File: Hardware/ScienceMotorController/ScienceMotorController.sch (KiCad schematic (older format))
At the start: 0 parts

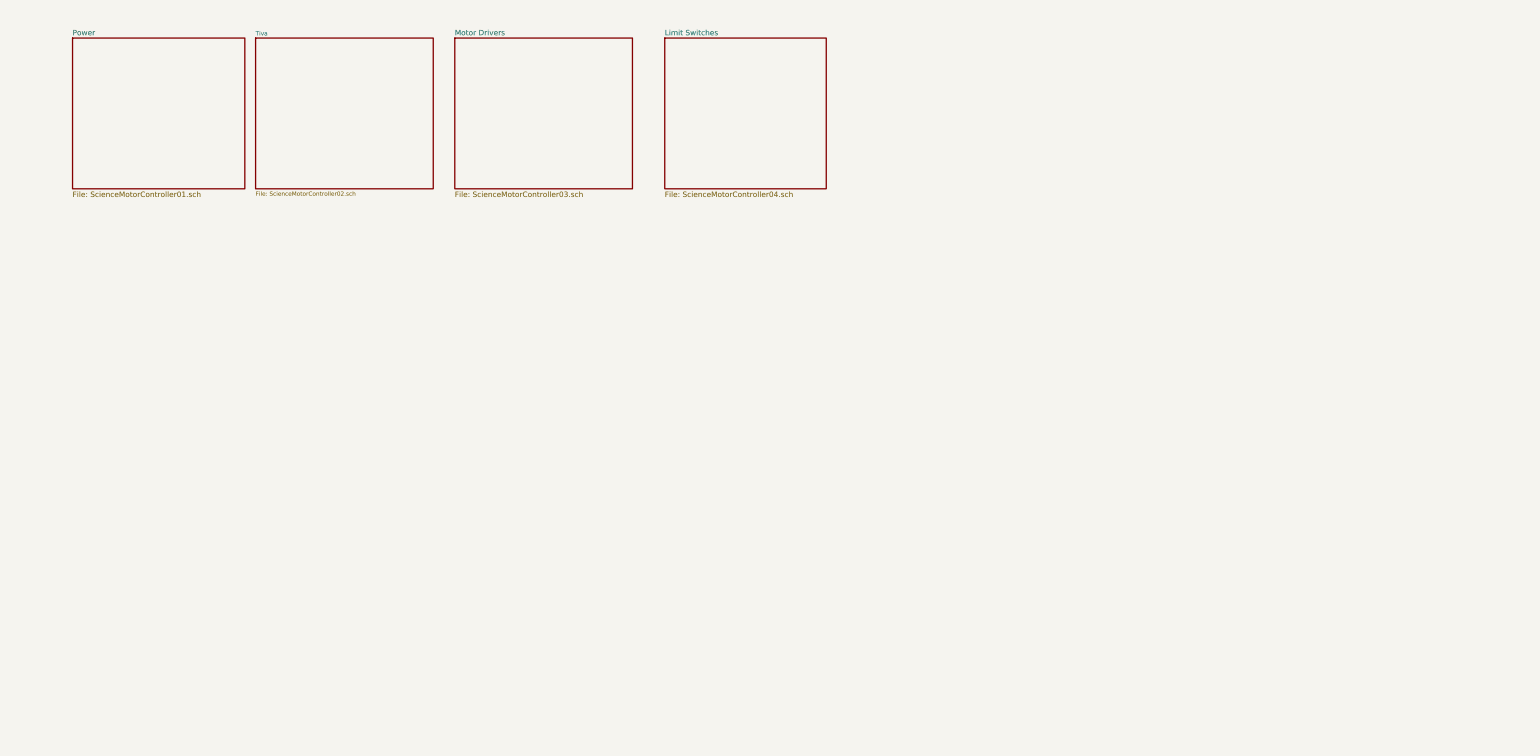
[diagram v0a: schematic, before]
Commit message: schematic review
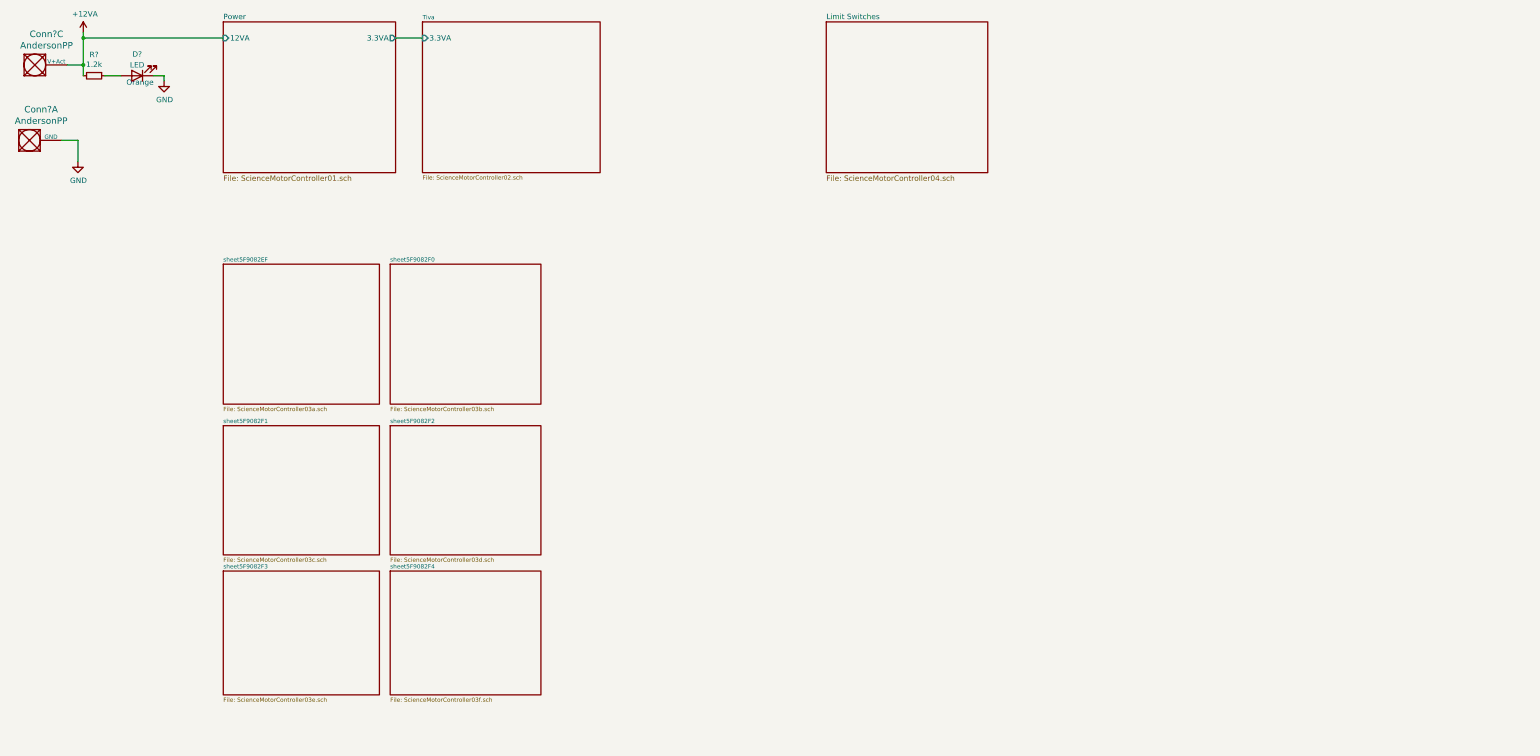
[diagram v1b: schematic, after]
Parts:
- added Conn? (x2): AndersonPP, symbol MRDT_Connectors:AndersonPP
- added D?: LED, symbol Device:LED
- added R?: 1.2k, symbol Device:R_Small
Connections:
- new net: D?.2 (A), R?.1
- new net +12VA: Conn?.3 (V+Act), R?.2
- new net GND: Conn?.1 (GND), D?.1 (K)
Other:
- note added: "Orange"
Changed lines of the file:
@@
 $Descr A 11000 8500
 encoding utf-8
-Sheet 1 11
+Sheet 1 10
 Title ""
 Date ""
@@
 $EndDescr
 $Sheet
-S 1100 1050 1600 1400
+S 2500 900  1600 1400
 U 5F6E1E86
 F0 "Power" 50
 F1 "ScienceMotorController01.sch" 50
+F2 "12VA" I L 2500 1050 50
+F3 "3.3VA" O R 4100 1050 50
 $EndSheet
 $Sheet
-S 2800 1050 1650 1400
+S 4350 900  1650 1400
 U 5F7148FA
 F0 "Tiva" 39
 F1 "ScienceMotorController02.sch" 39
+F2 "3.3VA" I L 4350 1050 50
 $EndSheet
 $Sheet
-S 4650 1050 1650 1400
-U 5F7D111E
-F0 "Motor Drivers" 50
-F1 "ScienceMotorController03.sch" 50
-$EndSheet
-$Sheet
-S 6600 1050 1500 1400
+S 8100 900  1500 1400
 U 5F81B171
 F0 "Limit Switches" 50
 F1 "ScienceMotorController04.sch" 50
 $EndSheet
+$Comp
+L MRDT_Connectors:AndersonPP Conn?
+U 3 1 5F8E3C0A
+P 650 1400
+AR Path="/5F6E1E86/5F8E3C0A" Ref="Conn?"  Part="3"
+AR Path="/5F8E3C0A" Ref="Conn?"  Part="3"
+F 0 "Conn?" H 858 1787 60  0000 C CNN
+F 1 "AndersonPP" H 858 1681 60  0000 C CNN
+F 2 "" H 500 850 60  0001 C CNN
+F 3 "" H 500 850 60  0001 C CNN
+	3    650  1400
+	1    0    0    -1
+$EndComp
+Wire Wire Line
+	1050 1300 1200 1300
+$Comp
+L power:+12VA #PWR?
+U 1 1 5F8E3C12
+P 1200 1000
+AR Path="/5F6E1E86/5F8E3C12" Ref="#PWR?"  Part="1"
+AR Path="/5F8E3C12" Ref="#PWR?"  Part="1"
+F 0 "#PWR?" H 1200 850 50  0001 C CNN
+F 1 "+12VA" H 1215 1173 50  0000 C CNN
+F 2 "" H 1200 1000 50  0001 C CNN
+F 3 "" H 1200 1000 50  0001 C CNN
+	1    1200 1000
+	1    0    0    -1
+$EndComp
+$Comp
+L Device:LED D?
+U 1 1 5F8E3C18
+P 1700 1400
+AR Path="/5F6E1E86/5F8E3C18" Ref="D?"  Part="1"
+AR Path="/5F8E3C18" Ref="D?"  Part="1"
+F 0 "D?" H 1700 1200 50  0000 C CNN
+F 1 "LED" H 1700 1300 50  0000 C CNN
+F 2 "" H 1700 1400 50  0001 C CNN
+F 3 "~" H 1700 1400 50  0001 C CNN
+	1    1700 1400
+	-1   0    0    1
+$EndComp
+Wire Wire Line
+	1200 1400 1200 1300
+Connection ~ 1200 1300
+$Comp
+L Device:R_Small R?
+U 1 1 5F8E3C20
+P 1300 1400
+AR Path="/5F6E1E86/5F8E3C20" Ref="R?"  Part="1"
+AR Path="/5F8E3C20" Ref="R?"  Part="1"
+F 0 "R?" V 1104 1400 50  0000 C CNN
+F 1 "1.2k" V 1195 1400 50  0000 C CNN
+F 2 "" H 1300 1400 50  0001 C CNN
+F 3 "~" H 1300 1400 50  0001 C CNN
+	1    1300 1400
+	0    1    1    0
+$EndComp
+Wire Wire Line
+	1400 1400 1550 1400
+$Comp
+L power:GND #PWR?
+U 1 1 5F8E3C27
+P 1950 1450
+AR Path="/5F6E1E86/5F8E3C27" Ref="#PWR?"  Part="1"
+AR Path="/5F8E3C27" Ref="#PWR?"  Part="1"
+F 0 "#PWR?" H 1950 1200 50  0001 C CNN
+F 1 "GND" H 1955 1277 50  0000 C CNN
+F 2 "" H 1950 1450 50  0001 C CNN
+F 3 "" H 1950 1450 50  0001 C CNN
+	1    1950 1450
+	1    0    0    -1
+$EndComp
+Wire Wire Line
+	1850 1400 1950 1400
+Wire Wire Line
+	1950 1400 1950 1450
+Text Notes 1600 1500 0    50   ~ 0
+Orange
+Wire Wire Line
+	1200 1050 1200 1300
+Wire Wire Line
+	2500 1050 1200 1050
+Connection ~ 1200 1050
+Wire Wire Line
+	1200 1000 1200 1050
+$Comp
+L MRDT_Connectors:AndersonPP Conn?
+U 1 1 5F8FDE30
+P 600 2100
+AR Path="/5F6E1E86/5F8FDE30" Ref="Conn?"  Part="1"
+AR Path="/5F8FDE30" Ref="Conn?"  Part="1"
+F 0 "Conn?" H 808 2487 60  0000 C CNN
+F 1 "AndersonPP" H 808 2381 60  0000 C CNN
+F 2 "" H 450 1550 60  0001 C CNN
+F 3 "" H 450 1550 60  0001 C CNN
+	1    600  2100
+	1    0    0    -1
+$EndComp
+$Comp
+L power:GND #PWR?
+U 1 1 5F8FDE36
+P 1150 2200
+AR Path="/5F6E1E86/5F8FDE36" Ref="#PWR?"  Part="1"
+AR Path="/5F8FDE36" Ref="#PWR?"  Part="1"
+F 0 "#PWR?" H 1150 1950 50  0001 C CNN
+F 1 "GND" H 1155 2027 50  0000 C CNN
+F 2 "" H 1150 2200 50  0001 C CNN
+F 3 "" H 1150 2200 50  0001 C CNN
+	1    1150 2200
+	1    0    0    -1
+$EndComp
+Wire Wire Line
+	1150 2200 1150 2000
+Wire Wire Line
+	1150 2000 1000 2000
+Wire Wire Line
+	4100 1050 4350 1050
+$Sheet
+S 2500 3150 1450 1300
+U 5F9082F6
+F0 "sheet5F9082EF" 39
+F1 "ScienceMotorController03a.sch" 39
+$EndSheet
+$Sheet
+S 4050 3150 1400 1300
+U 5F9082F8
+F0 "sheet5F9082F0" 39
+F1 "ScienceMotorController03b.sch" 39
+$EndSheet
+$Sheet
+S 2500 4650 1450 1200
+U 5F9082FA
+F0 "sheet5F9082F1" 39
+F1 "ScienceMotorController03c.sch" 39
+$EndSheet
+$Sheet
+S 4050 4650 1400 1200
+U 5F9082FC
+F0 "sheet5F9082F2" 39
+F1 "ScienceMotorController03d.sch" 39
+$EndSheet
+$Sheet
+S 2500 6000 1450 1150
+U 5F9082FE
+F0 "sheet5F9082F3" 39
+F1 "ScienceMotorController03e.sch" 39
+$EndSheet
+$Sheet
+S 4050 6000 1400 1150
+U 5F908300
+F0 "sheet5F9082F4" 39
+F1 "ScienceMotorController03f.sch" 39
+$EndSheet
 $EndSCHEMATC

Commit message: made some more hierarchal changes
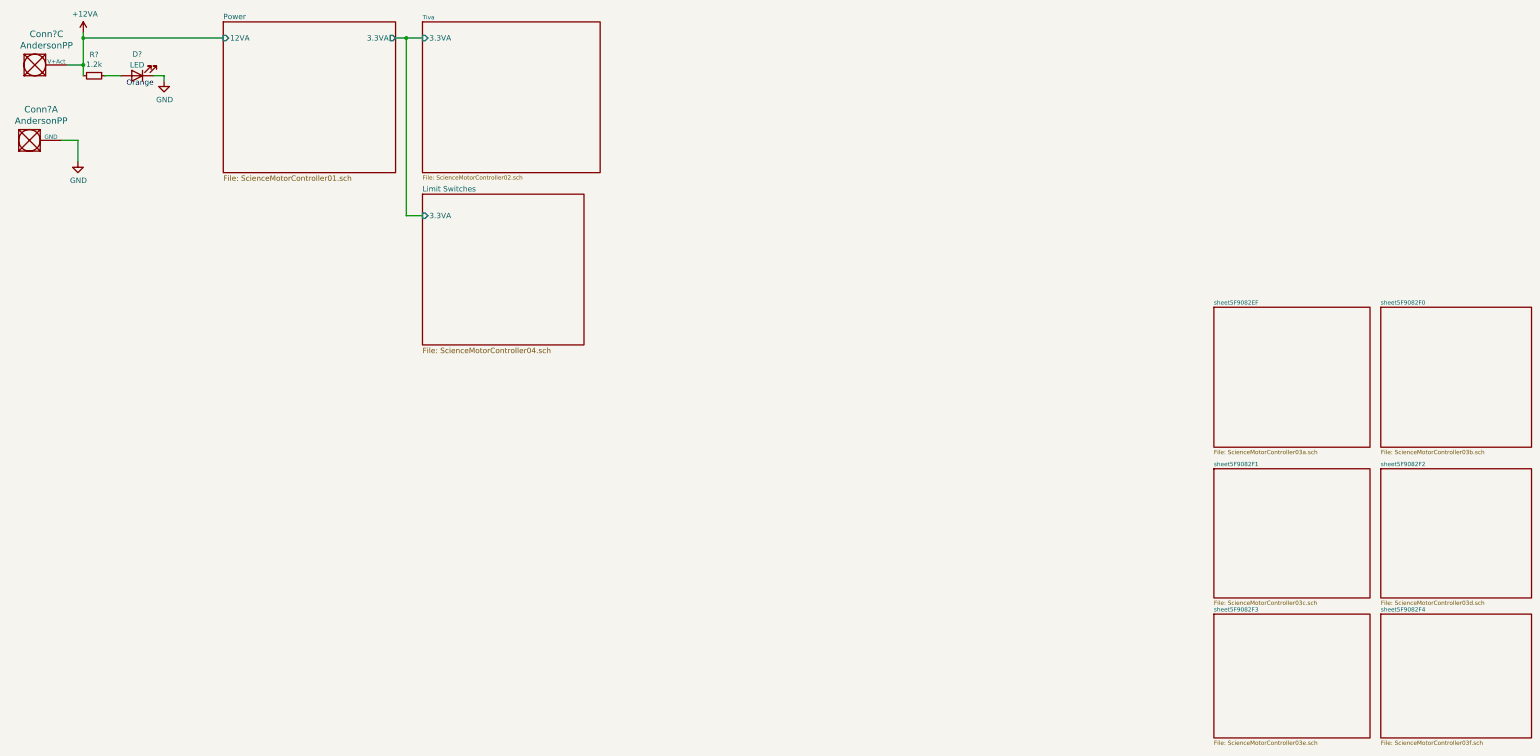
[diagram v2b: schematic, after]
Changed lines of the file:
@@
 $EndSheet
 $Sheet
-S 8100 900  1500 1400
+S 4350 2500 1500 1400
 U 5F81B171
 F0 "Limit Switches" 50
 F1 "ScienceMotorController04.sch" 50
+F2 "3.3VA" I L 4350 2700 50
 $EndSheet
 $Comp
@@
 	1150 2000 1000 2000
 Wire Wire Line
-	4100 1050 4350 1050
+	4100 1050 4200 1050
 $Sheet
-S 2500 3150 1450 1300
+S 11700 3550 1450 1300
 U 5F9082F6
 F0 "sheet5F9082EF" 39
@@
 $EndSheet
 $Sheet
-S 4050 3150 1400 1300
+S 13250 3550 1400 1300
 U 5F9082F8
 F0 "sheet5F9082F0" 39
@@
 $EndSheet
 $Sheet
-S 2500 4650 1450 1200
+S 11700 5050 1450 1200
 U 5F9082FA
 F0 "sheet5F9082F1" 39
@@
 $EndSheet
 $Sheet
-S 4050 4650 1400 1200
+S 13250 5050 1400 1200
 U 5F9082FC
 F0 "sheet5F9082F2" 39
@@
 $EndSheet
 $Sheet
-S 2500 6000 1450 1150
+S 11700 6400 1450 1150
 U 5F9082FE
 F0 "sheet5F9082F3" 39
@@
 $EndSheet
 $Sheet
-S 4050 6000 1400 1150
+S 13250 6400 1400 1150
 U 5F908300
 F0 "sheet5F9082F4" 39
 F1 "ScienceMotorController03f.sch" 39
 $EndSheet
+Wire Wire Line
+	4350 2700 4200 2700
+Wire Wire Line
+	4200 2700 4200 1050
+Connection ~ 4200 1050
+Wire Wire Line
+	4200 1050 4350 1050
 $EndSCHEMATC
